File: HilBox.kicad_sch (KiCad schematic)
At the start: 4 parts

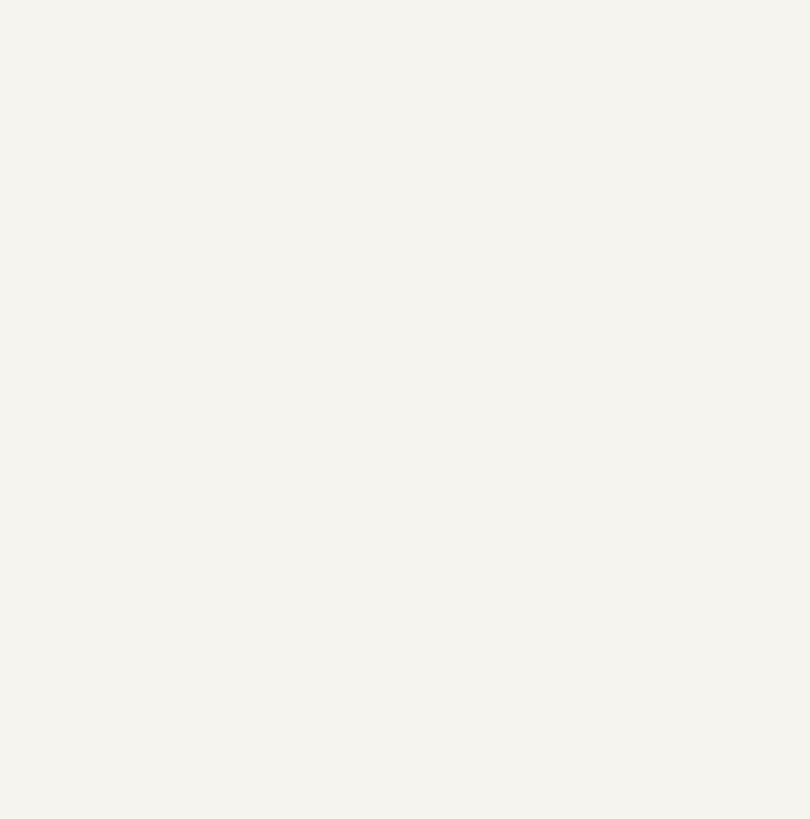
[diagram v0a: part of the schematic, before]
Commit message: Schematic design at finish
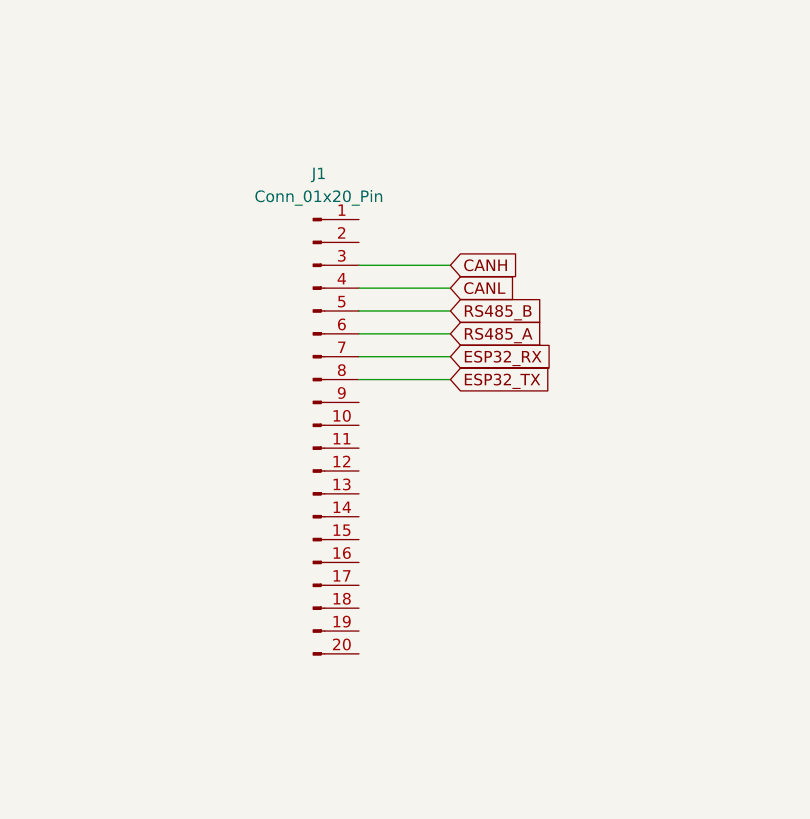
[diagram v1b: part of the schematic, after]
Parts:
- added J1: Conn_01x20_Pin, Connectors:Terminal_Block_3_81_20p_Horizontal, symbol Connector:Conn_01x20_Pin
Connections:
- new net CANH: J1.3 (Pin_3)
- new net CANL: J1.4 (Pin_4)
- new net ESP32_RX: J1.7 (Pin_7)
- new net ESP32_TX: J1.8 (Pin_8)
- new net RS485_A: J1.6 (Pin_6)
- new net RS485_B: J1.5 (Pin_5)

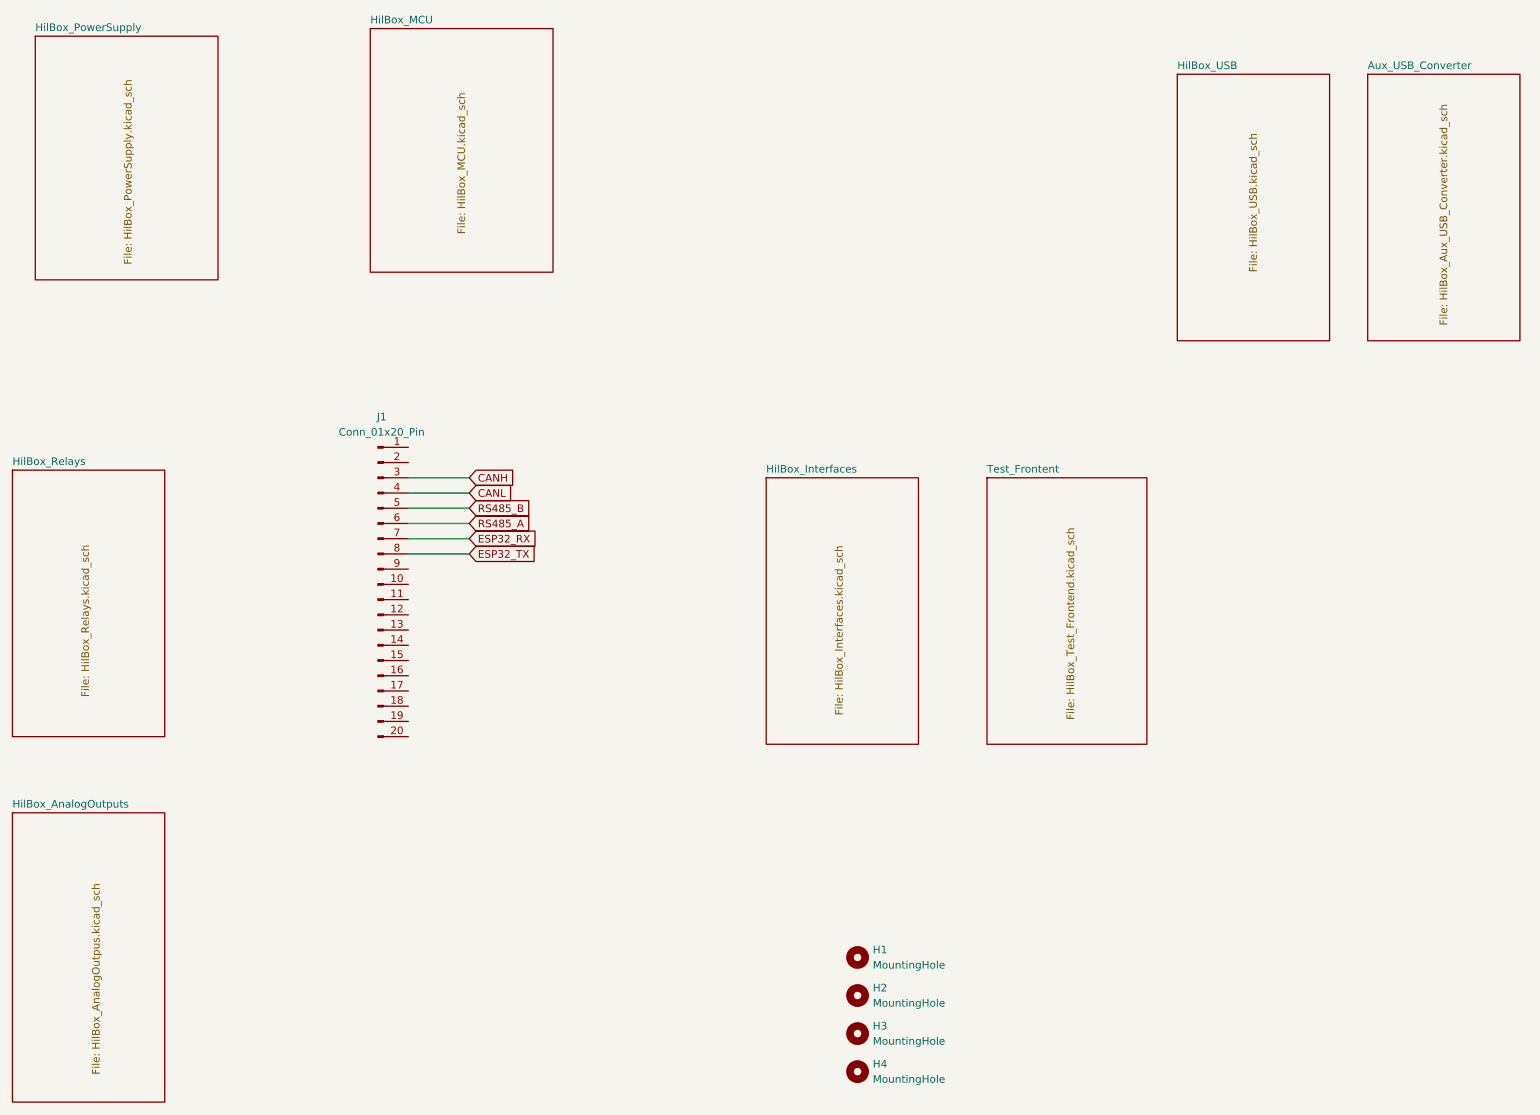
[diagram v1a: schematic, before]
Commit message: Layout 90% done
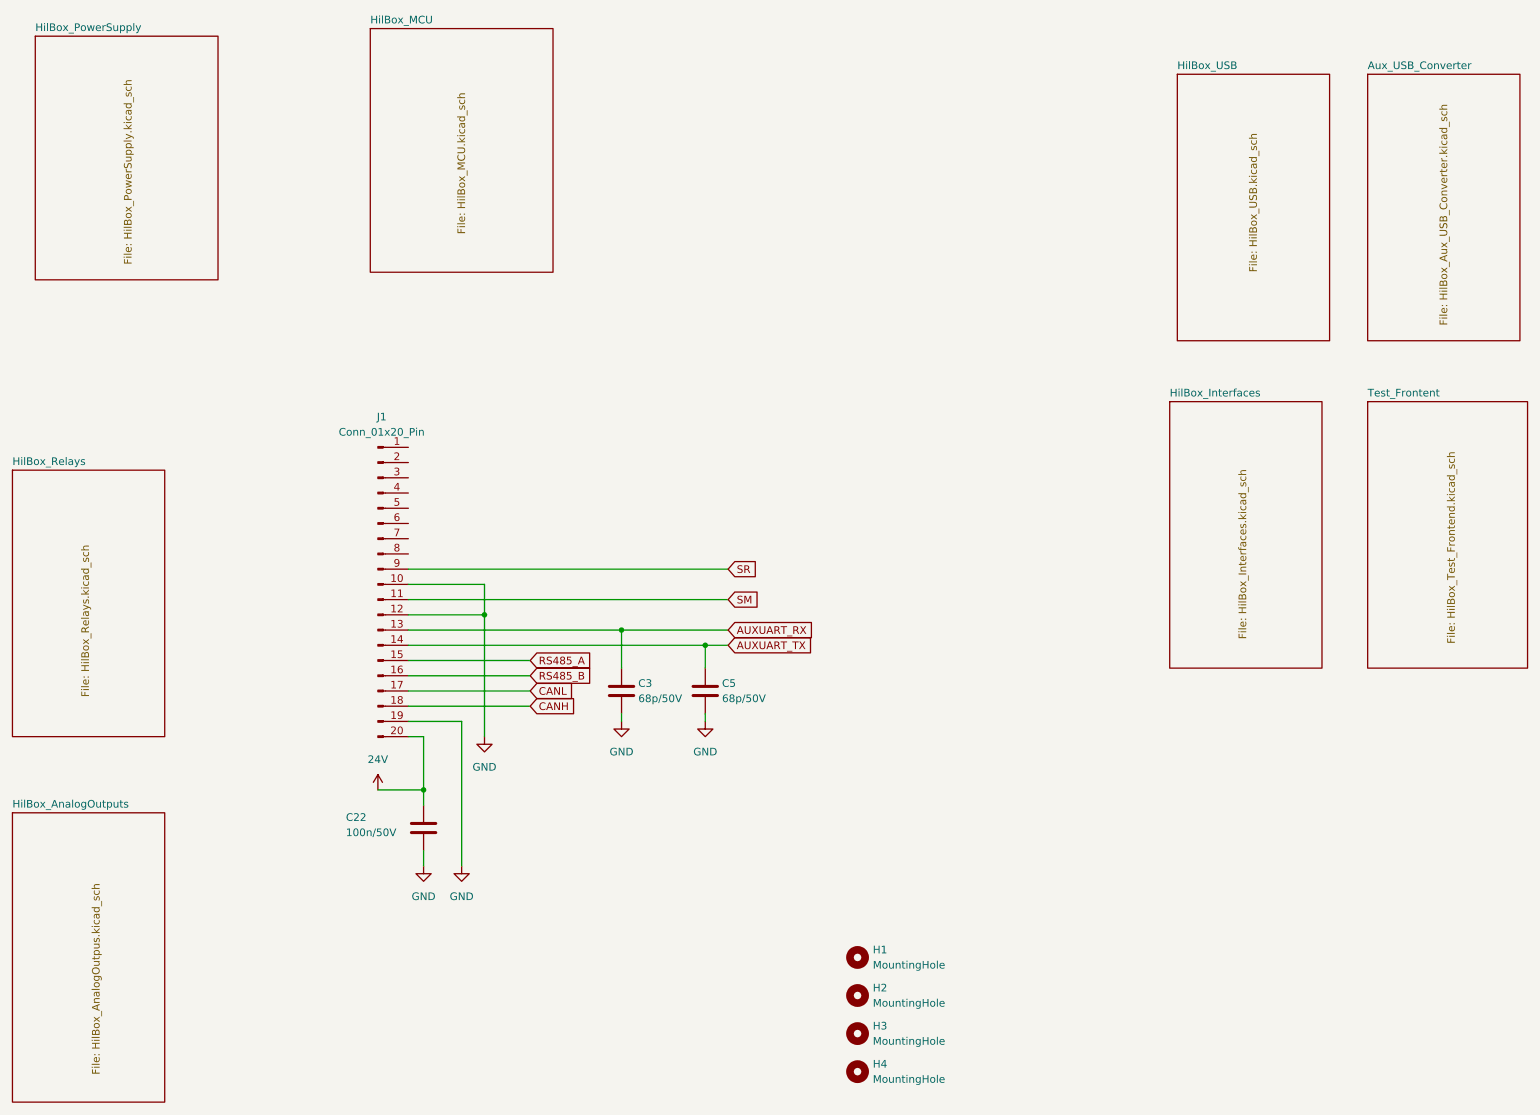
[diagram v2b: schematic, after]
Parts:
- added C22: 100n/50V, Capacitor_SMD:C_0402_1005Metric, symbol Device:C
- added C3, C5: 68p/50V, Capacitor_SMD:C_0402_1005Metric, symbol Device:C
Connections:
- net CANH: now also J1.18 (Pin_18); no longer J1.3 (Pin_3)
- net CANL: now also J1.17 (Pin_17); no longer J1.4 (Pin_4)
- net RS485_A: now also J1.15 (Pin_15); no longer J1.6 (Pin_6)
- net RS485_B: now also J1.16 (Pin_16); no longer J1.5 (Pin_5)
- net GND: now reaches J1.10 (Pin_10)
- net GND: now also J1.12 (Pin_12), J1.19 (Pin_19), C22.2, C3.2, C5.2
- net SM: now reaches J1.11 (Pin_11)
- net AUXUART_RX: now reaches J1.13 (Pin_13)
- net AUXUART_RX: now also C3.1
- net AUXUART_TX: now reaches J1.14 (Pin_14)
- net AUXUART_TX: now also C5.1
- net 24V: now reaches J1.20 (Pin_20)
- net 24V: now also C22.1
- net SR: now reaches J1.9 (Pin_9)
- net ESP32_RX: no longer names the net of J1.7 (Pin_7)
- net ESP32_TX: no longer names the net of J1.8 (Pin_8)
